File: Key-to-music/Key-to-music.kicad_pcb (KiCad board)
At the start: 2 copper layers, 21 x 21 mm, 62 parts, among them J1 USB_C_Receptacle_USB2.0_16P, SW1 B3U1000P, SW2 SW_Push, SW3 SW_Push, U1 AP1117-33, U2 W25Q128JVS, U3 RP2040, Y1 Crystal_GND24

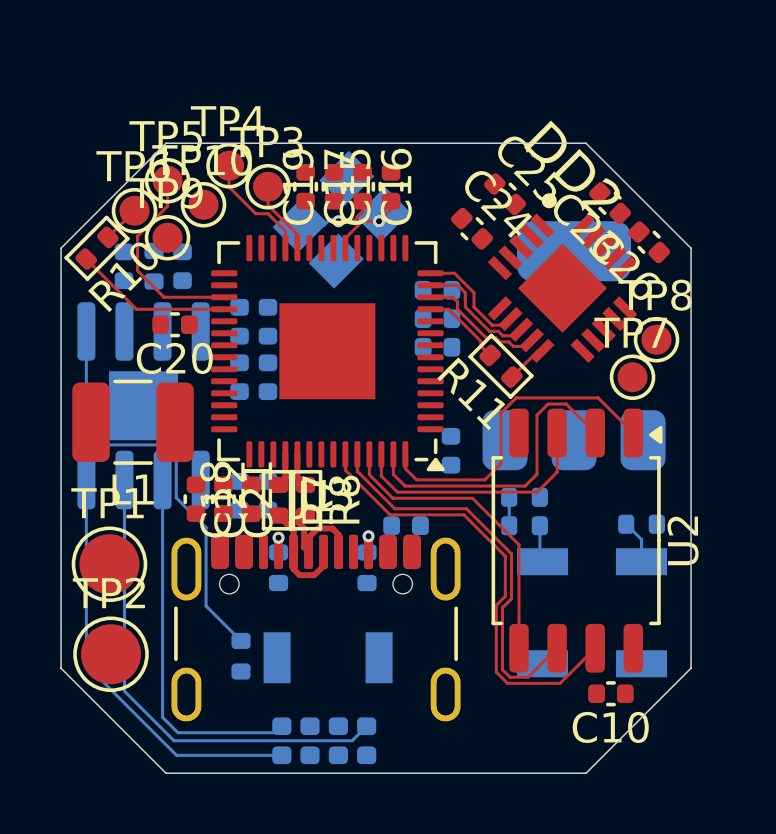
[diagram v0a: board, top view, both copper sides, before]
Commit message: rev0 готова
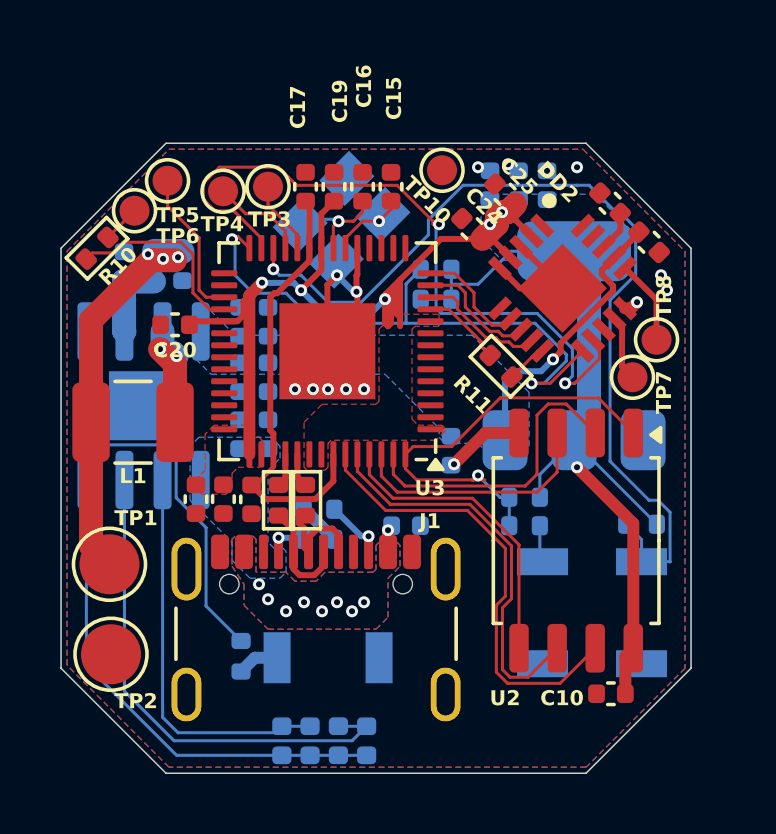
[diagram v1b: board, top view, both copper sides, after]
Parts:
- removed TP9: LED-, TestPoint:TestPoint_Pad_D1.0mm
- added G***: LOGO, LOGO, B.Cu at (158.6, 114.8)
- added R12: 10K, PCM_Resistor_SMD_AKL:R_0402_1005Metric, B.Cu at (169.0, 103.2)
- added R13: 10K, PCM_Resistor_SMD_AKL:R_0402_1005Metric, B.Cu at (169.0, 104.2)
- moved TP10 8.03 mm to (169.2, 99.9)
- moved C6 5.68 mm to (170.8, 100.4), turned to 90 degrees
- moved C4 5.21 mm to (171.8, 100.4), turned to 90 degrees
- moved C5 5.06 mm to (172.7, 100.4), turned to 90 degrees
- moved R2 2.52 mm to (165.1, 111.2), turned to 180 degrees
- moved C2 2.26 mm to (163.4, 108.7), turned to 90 degrees
- moved C3 2.26 mm to (162.4, 108.7), turned to 90 degrees
- moved R1 1.65 mm to (165.1, 112.2), turned to 0 degrees
- moved TP4 0.87 mm to (161.9, 100.6)
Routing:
- net +3.3V: track 0.00 -> 59.6 mm, vias 0 -> 6
- net Net-(U3-RUN): track 1.46 -> 30.6 mm, vias 0 -> 1
- net SDA: track 0.00 -> 24.2 mm, vias 0 -> 2
- net SCL: track 0.00 -> 20.0 mm, vias 0 -> 2
- net Earth: track 0.00 -> 16.8 mm, vias 0 -> 15
- net Net-(U3-VREG_VOUT): track 0.00 -> 14.6 mm
- net Net-(C14-Pad1): track 0.00 -> 13.0 mm, vias 0 -> 3
- net +5V: track 0.00 -> 9.63 mm, vias 0 -> 1
- net Net-(DD1-SW): track 0.00 -> 3.75 mm, vias 0 -> 2
- net Net-(U2-~{CS}): track 11.8 -> 14.7 mm, vias 0 -> 1
- net Net-(D1-K): track 13.9 -> 16.8 mm
- net Net-(DD2-SPKOUT_-): track 0.00 -> 2.82 mm
- net Net-(DD1-BAT): track 0.00 -> 2.71 mm
- net Net-(DD2-SPKOUT+): track 0.00 -> 2.19 mm
- net +5V USB: track 0.00 -> 1.76 mm, vias 0 -> 9
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- added copper zone on B.Cu, net +3.3V
- added copper zone on F.Cu, net +3.3V
- added copper zone on B.Cu, net +5V
- added copper zone on B.Cu, net +5V USB
- added copper zone on F.Cu, net +5V USB
- added copper zone on B.Cu, net Earth
- added copper zone on F.Cu, net Earth
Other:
- board text added: "@madjogger"
- board text added: "Key to"
- board text added: "music"
- board text added: "мяу"
